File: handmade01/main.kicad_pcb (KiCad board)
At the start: 2 copper layers, 64.8 x 70.1 mm, 71 parts, among them CON1 MicroSD, CON2 MicroSD, J1 JACK_TRS_6PINS, P1 VOLUMN, P4 USB_OTG, P6 UART_DEBUG, Q1 1AM, SW1 Power, SW10 R, SW11 A, SW12 B, SW13 X, SW14 Y, SW2 Reset, SW3 UP, SW4 Down, SW5 Left, SW6 Right, SW7 Select, SW8 Start, SW9 L, U1 PCM5102A, U2 PAM8403, U3 IPS_2.4_240x320_ST7789V, U4 CM3354, U5 TPS71718

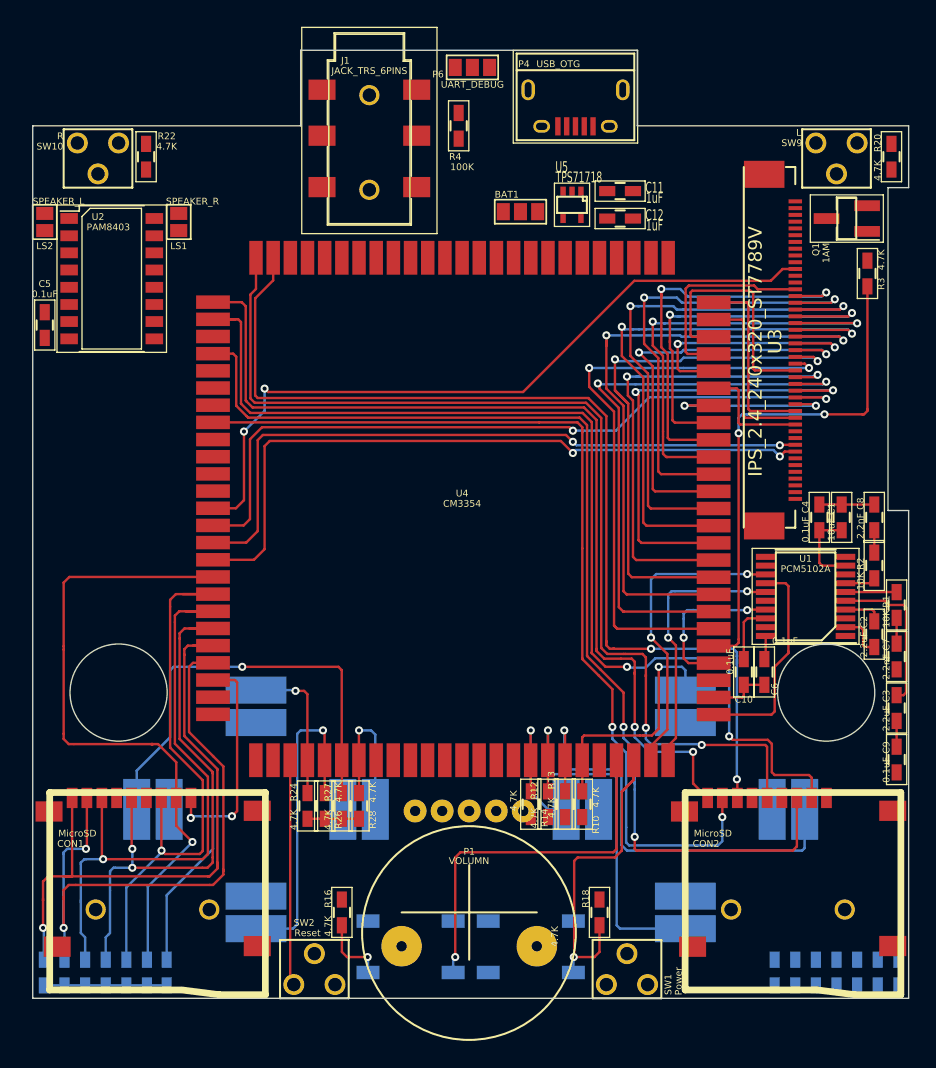
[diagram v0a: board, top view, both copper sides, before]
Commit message: 20171216
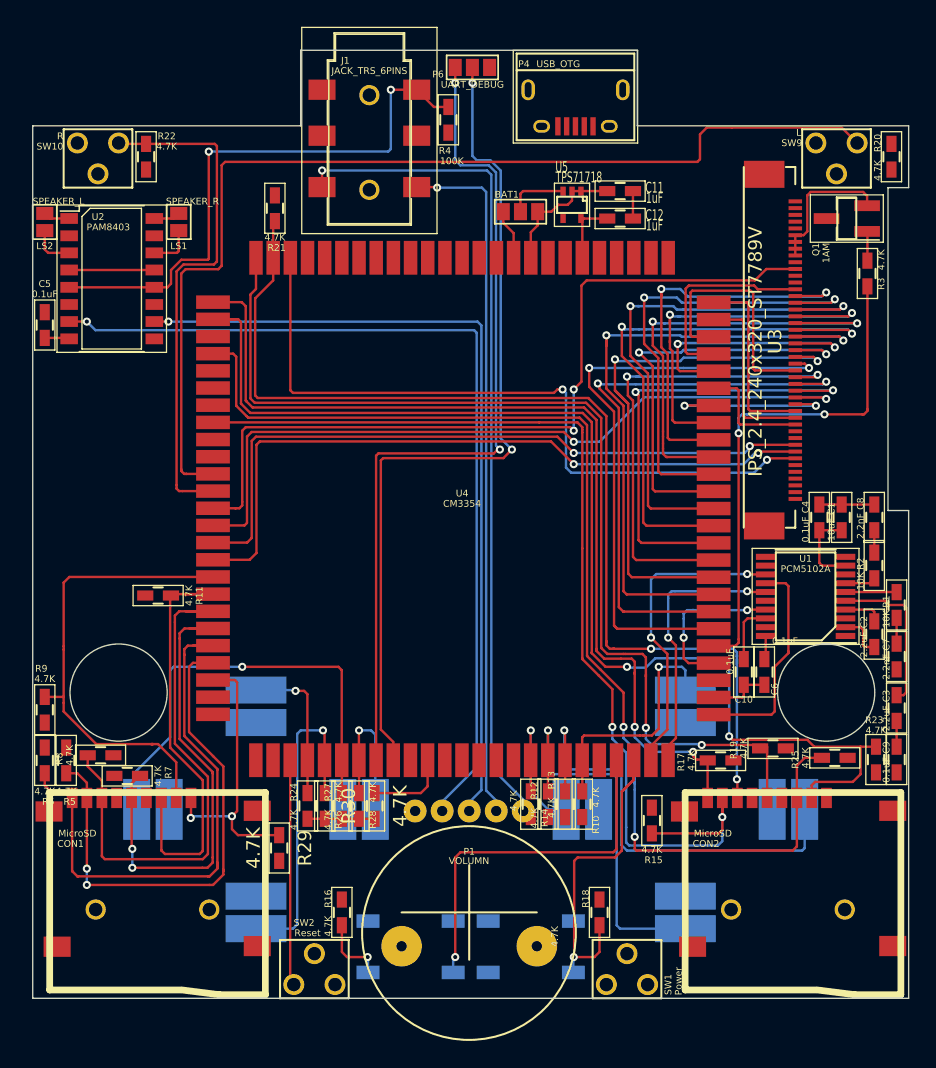
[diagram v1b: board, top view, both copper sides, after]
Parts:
- R11, R15, R17, R19, R21, R23, R25, R29, R30, R5, R6, R7, R8, R9: moved to F.Cu
- moved R21 70.1 mm to (128.4, 79.2), turned to 270 degrees
- moved R30 32.1 mm to (135.8, 123.4)
- moved R11 28.0 mm to (119.8, 107.9), turned to 0 degrees
- moved R9 20.8 mm to (111.4, 116.3)
- moved R19 17.7 mm to (165.2, 119.2), turned to 180 degrees
- moved R17 16.6 mm to (161.4, 120.1), turned to 180 degrees
- moved R15 16.5 mm to (156.3, 124.5), turned to 270 degrees
- moved R25 16.2 mm to (169.8, 119.9), turned to 180 degrees
- moved R8 16.1 mm to (115.5, 119.7), turned to 180 degrees
- moved R23 15.8 mm to (172.8, 120.0)
- moved R5 15.7 mm to (113.0, 120.1), turned to 270 degrees
- moved R6 15.7 mm to (111.4, 120.1), turned to 270 degrees
- moved R7 14.6 mm to (117.5, 121.2), turned to 0 degrees
- moved R29 12.4 mm to (128.7, 126.6)
- moved R4 0.88 mm to (141.2, 72.7)
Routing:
- net L: track 0.00 -> 77.4 mm
- net INL: track 0.00 -> 66.9 mm, vias 0 -> 1
- net UART_RX: track 0.00 -> 62.7 mm, vias 0 -> 2
- net UART_TX: track 0.00 -> 62.6 mm, vias 0 -> 2
- net OUTL: track 1.91 -> 63.8 mm, vias 0 -> 1
- net INR: track 0.00 -> 60.6 mm, vias 0 -> 1
- net LCD_RESET: track 0.00 -> 53.5 mm, vias 0 -> 2
- net OUTR: track 1.66 -> 53.0 mm, vias 0 -> 1
- net MUTE: track 0.00 -> 42.4 mm, vias 0 -> 2
- net R: track 0.00 -> 38.0 mm
- net SD0_DAT1: track 48.8 -> 35.2 mm, vias 1 -> 0
- net LED_K: track 0.00 -> 10.5 mm
- net BAT_+: track 0.00 -> 9.81 mm
- net SD0_DAT0: track 41.5 -> 32.3 mm, vias 1 -> 0
- net SD0_DAT3: track 47.2 -> 38.2 mm
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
